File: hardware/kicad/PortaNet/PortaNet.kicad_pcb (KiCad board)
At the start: 2 copper layers, 47.5 x 16.8 mm, 34 parts, among them J1 UART, J2 Molex 0480370001, J3 OLED_PINS, J4 GRPB052VWVN-RC, U1 ESP32-C3, U2 AP2114HA-3.3TRG1, Y1 FL400WFQA1

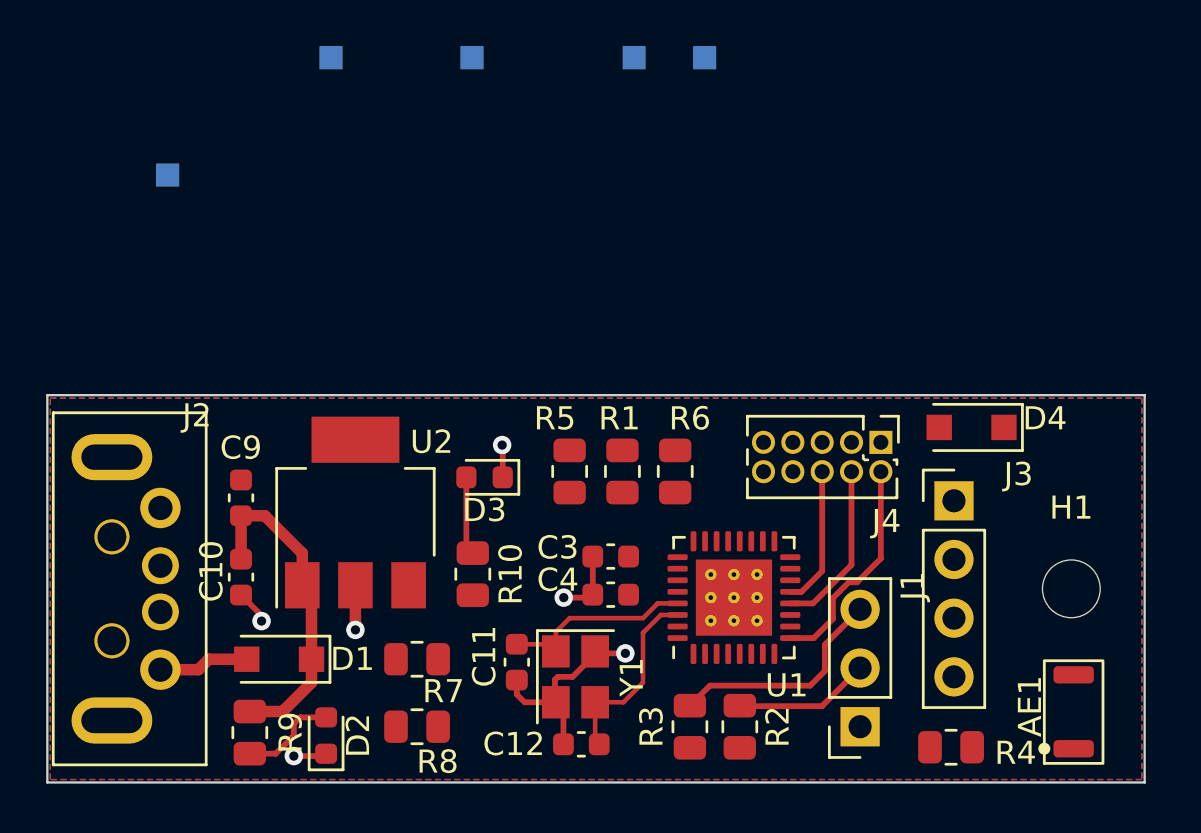
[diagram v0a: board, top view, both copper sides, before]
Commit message: first layout rev
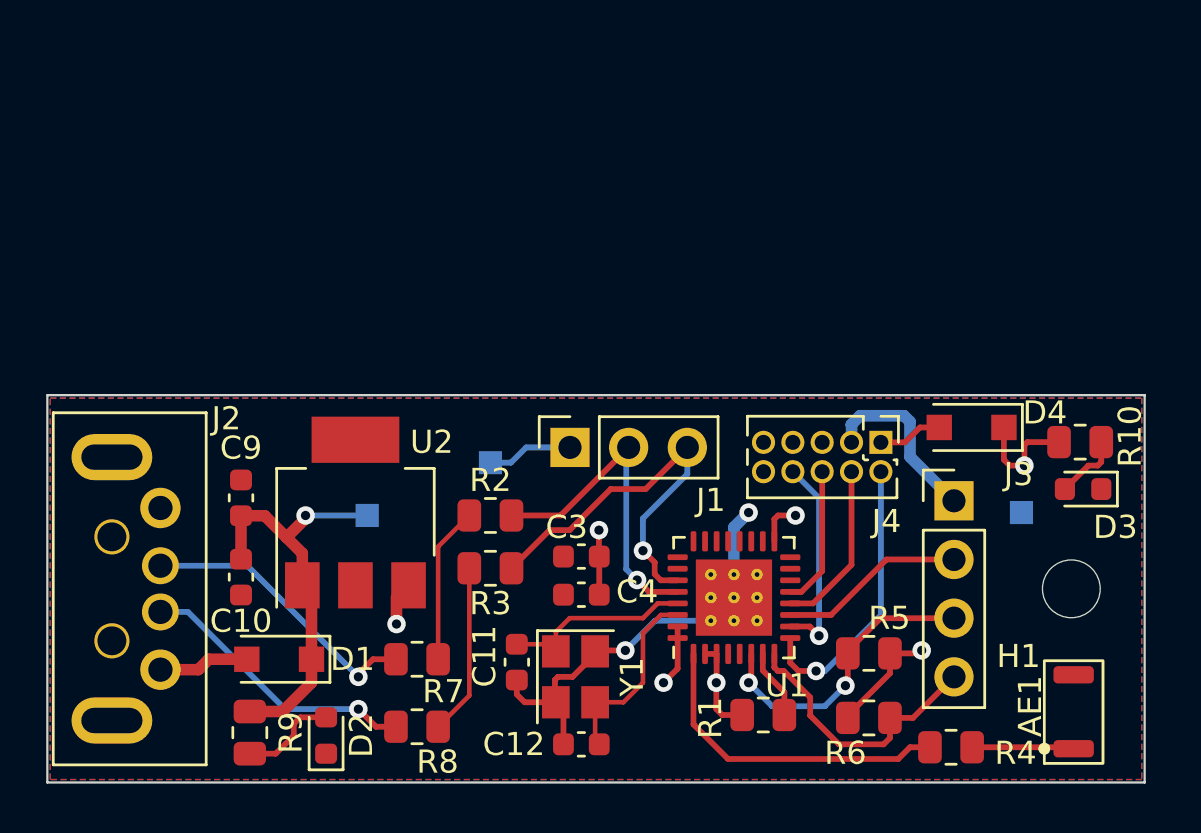
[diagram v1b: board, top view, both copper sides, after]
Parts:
- removed TP1, TP2: TestPoint, TestPoint:TestPoint_Pad_1.0x1.0mm
- moved TP4 39.7 mm to (163.8, 67.8)
- moved R10 26.9 mm to (166.4, 64.8), turned to 180 degrees
- moved D3 25.9 mm to (166.5, 66.8)
- moved TP3 20.3 mm to (135.5, 67.9), turned to -90 degrees
- moved TP5 18.8 mm to (140.8, 65.7)
- moved J1 17.4 mm to (144.3, 65.0), turned to 90 degrees
- moved R5 15.2 mm to (157.2, 73.9), turned to 0 degrees
- moved R2 14.1 mm to (140.8, 67.9), turned to 180 degrees
- moved R6 13.6 mm to (157.2, 76.7), turned to 180 degrees
- moved R1 12.2 mm to (152.7, 76.6), turned to 180 degrees
- moved R3 11.0 mm to (140.8, 70.2), turned to 0 degrees
- moved C3 1.27 mm to (144.8, 69.7)
- moved C4 1.27 mm to (144.8, 71.4)
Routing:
- net 3V3: track 0.00 -> 31.3 mm, vias 0 -> 7
- net Net-(R4-Pad2): track 0.00 -> 14.1 mm
- net I2C_SCL: track 0.00 -> 13.0 mm, vias 0 -> 2
- net Net-(J2-Pad3): track 0.00 -> 12.6 mm, vias 0 -> 1
- net Net-(J2-Pad2): track 0.00 -> 12.3 mm, vias 0 -> 1
- net I2C_SDA: track 0.00 -> 11.9 mm
- net GND: track 18.3 -> 27.9 mm, vias 6 -> 2
- net JTAG_TDI: track 0.00 -> 8.98 mm, vias 0 -> 1
- net Net-(J1-Pad2): track 5.90 -> 14.2 mm, vias 0 -> 1
- net Net-(J1-Pad3): track 9.76 -> 17.4 mm, vias 0 -> 1
- net USB_DN: track 0.00 -> 7.42 mm
- net USB_DP: track 0.00 -> 6.78 mm
- net ANT: track 0.00 -> 4.42 mm
- net 5V: track 14.2 -> 18.1 mm, vias 0 -> 1
- net Net-(R1-Pad1): track 0.00 -> 3.03 mm
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- added copper zone on B.Cu, net 3V3
- added copper zone on F.Cu, net GND
- removed copper zone on F.Cu, net 3V3
- removed copper zone on B.Cu, net GND
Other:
- board text added: "PortaNet v1.0, A JCM Design"
